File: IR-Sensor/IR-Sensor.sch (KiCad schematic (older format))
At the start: 11 parts

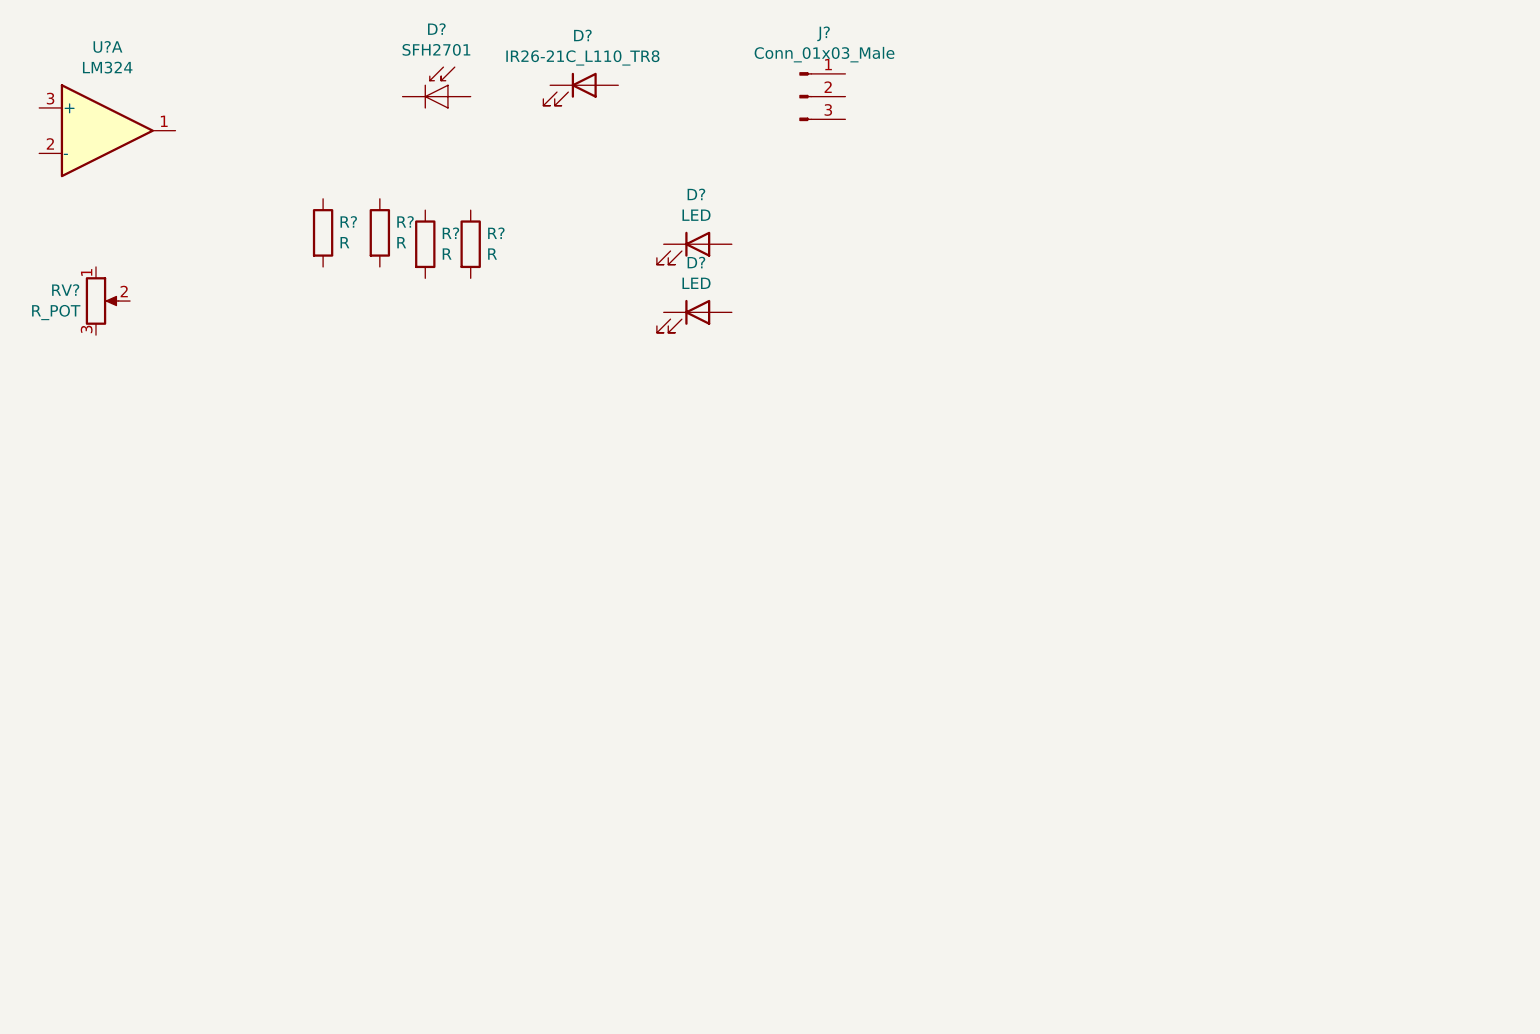
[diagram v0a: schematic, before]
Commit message: Added footprint & netlist
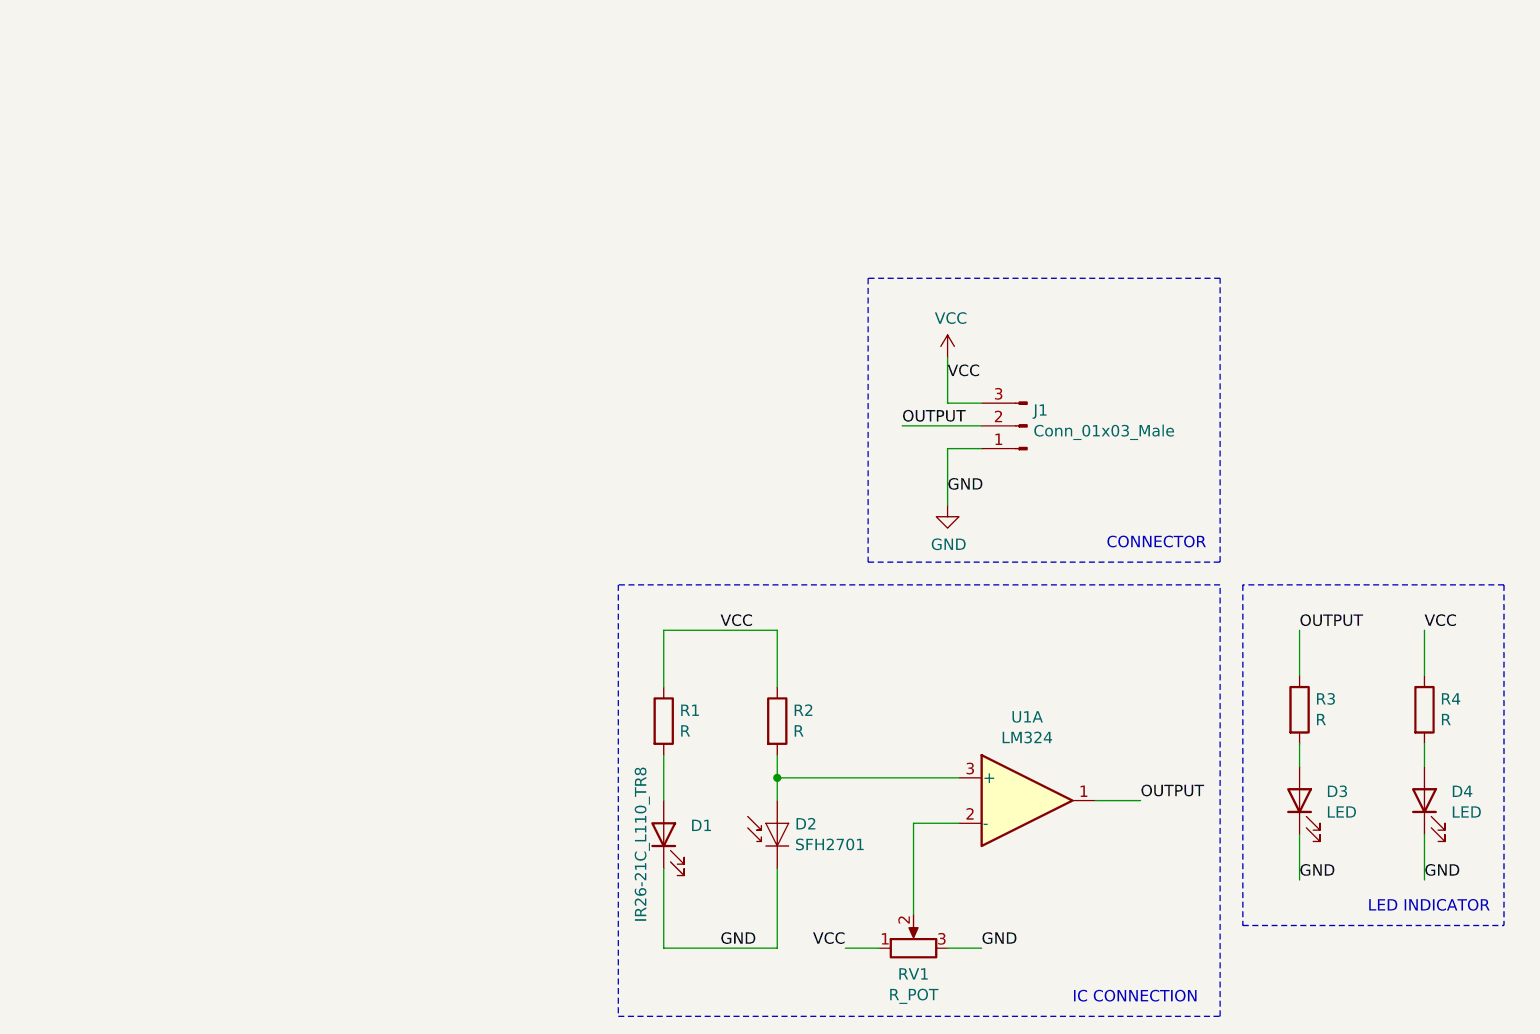
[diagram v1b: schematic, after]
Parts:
- removed D?: LED, symbol Device:LED
- removed R?: R, symbol Device:R
- added D3: LED, LED_SMD:LED_0805_2012Metric, symbol Device:LED
- added R3: R, Resistor_SMD:R_0805_2012Metric, symbol Device:R
- D4: renamed from D?; footprint (none) -> LED_SMD:LED_0805_2012Metric
- J1: renamed from J?; footprint (none) -> Connector_PinHeader_2.54mm:PinHeader_1x03_P2.54mm_Horizontal
- R1, R2, R4: renamed from R?; footprint (none) -> Resistor_SMD:R_0805_2012Metric
- RV1: renamed from RV?; footprint (none) -> Potentiometer_SMD:Potentiometer_Bourns_3314J_Vertical
- U1: renamed from U?; footprint (none) -> Package_SO:TSSOP-14_4.4x5mm_P0.65mm
- gave numbers to parts that had none: 2
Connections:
- net GND: now reaches D4.1 (K)
- net GND: now also D1.1 (K), D2.1 (K), J1.1 (Pin_1), RV1.3, D3.1 (K)
- net at D4.2 (A): now also R4.2
- net VCC: now reaches R2.1
- net VCC: now also J1.3 (Pin_3), R1.1, R4.1, RV1.1
- net at R2.2: now also D2.2 (A), U1.3 (+)
- net at R1.2: now also D1.2 (A)
- net OUTPUT: now reaches U1.1
- net OUTPUT: now also J1.2 (Pin_2), R3.1
- net at U1.2 (-): now also RV1.2
- new net: D3.2 (A), R3.2
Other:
- note added: "CONNECTOR"
- note added: "IC CONNECTION"
- note added: "LED INDICATOR"
- moved on the sheet: D1, D2, D4, J1, R1, R2, R4, RV1, U1A
